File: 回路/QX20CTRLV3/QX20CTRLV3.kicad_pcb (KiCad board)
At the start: 2 copper layers, 56 x 47 mm, 26 parts, among them J1 VH_CAN, J2 VH_CAN, J3 VH_SRV1, J4 VH_SRV2, J5 USART, J6 I2C, J7 Conn_01x05, SW2 SW_SPDT, U1 BP5293-33, U2 STM32F303K8Tx, U3 SN65HVD232

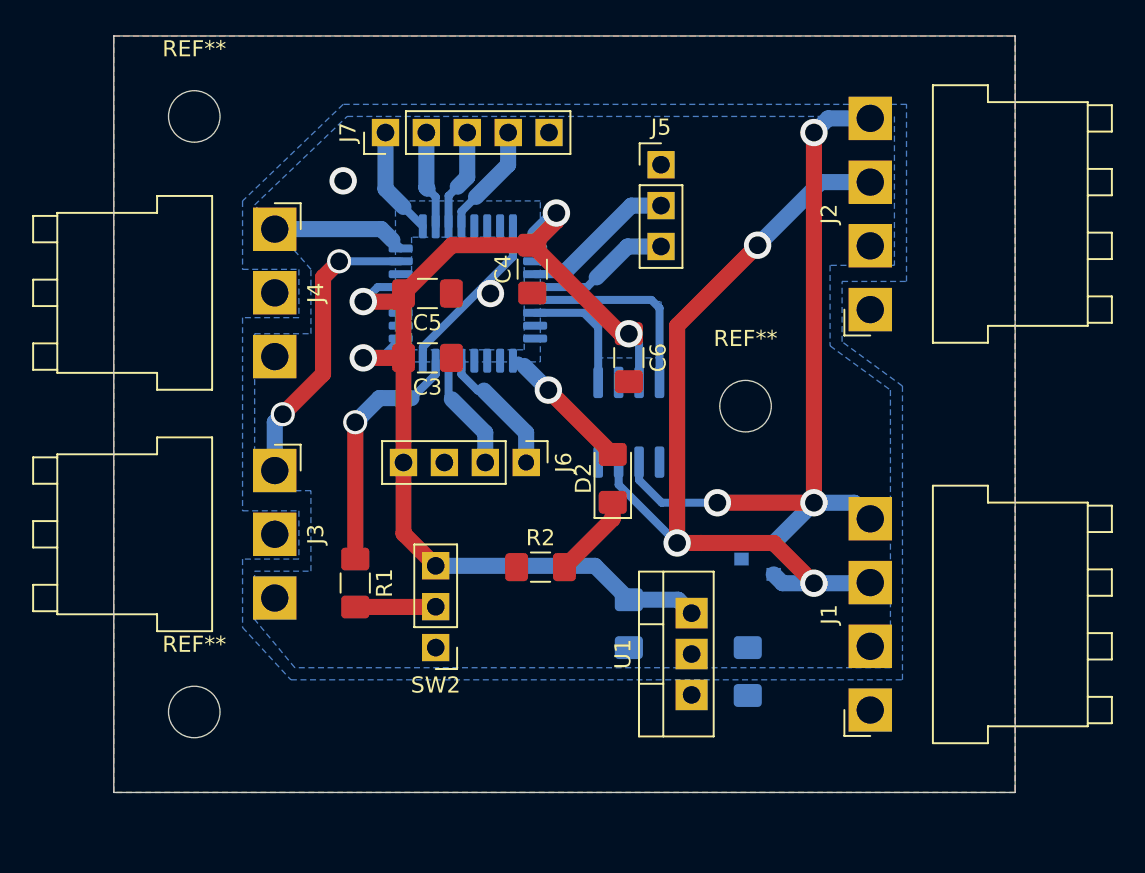
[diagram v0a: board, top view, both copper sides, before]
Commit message: QX20CTRLV3発注仕様
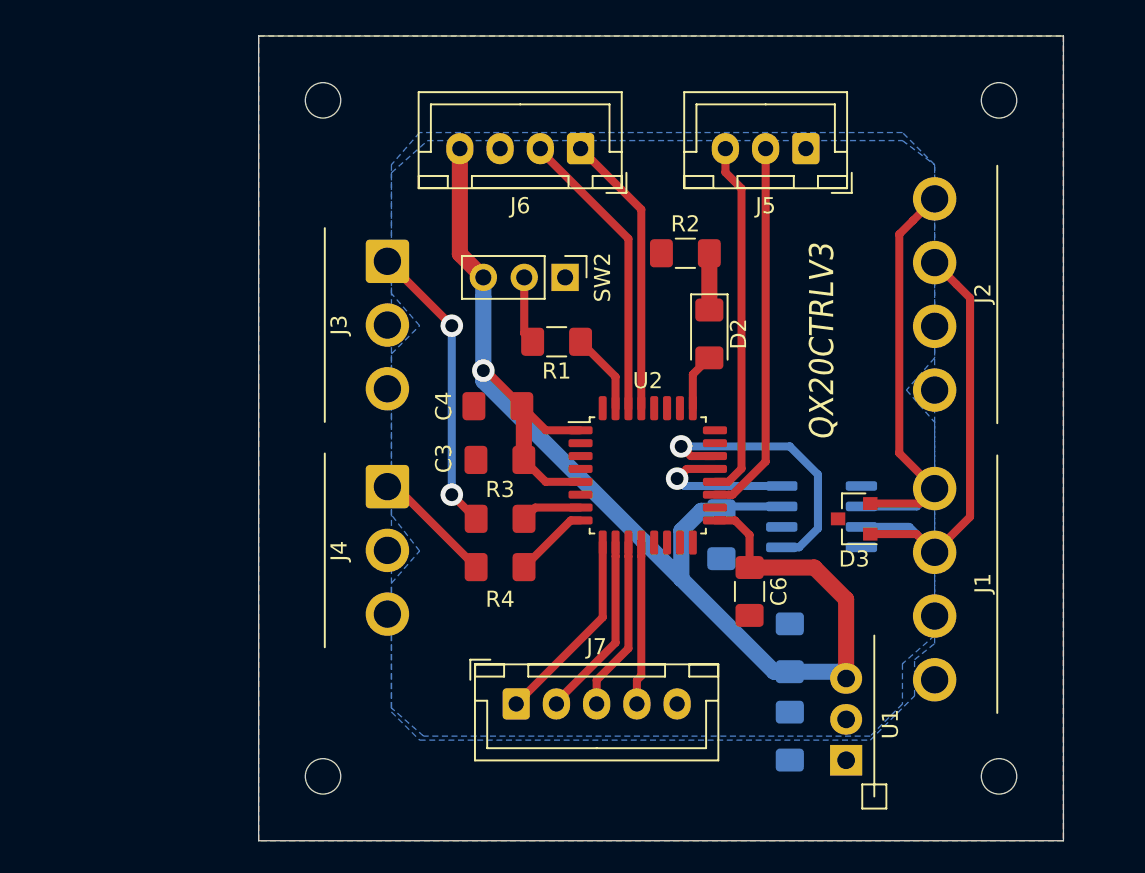
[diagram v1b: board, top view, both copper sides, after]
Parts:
- removed the ? at (151.0, 58.0)
- removed the ? at (152.0, 60.0)
- removed REF** (x3): MountingHole_3.2mm_M3, MountingHole:MountingHole_3.2mm_M3
- added ?: MountingHole_2.2mm_M2_DIN965, MountingHole:MountingHole_2.2mm_M2_DIN965, F.Cu at (104.0, 54.0)
- added ?: MountingHole_2.2mm_M2_DIN965, MountingHole:MountingHole_2.2mm_M2_DIN965, F.Cu at (104.0, 96.0)
- added ?: MountingHole_2.2mm_M2_DIN965, MountingHole:MountingHole_2.2mm_M2_DIN965, F.Cu at (146.0, 96.0)
- added ?: MountingHole_2.2mm_M2_DIN965, MountingHole:MountingHole_2.2mm_M2_DIN965, F.Cu at (146.0, 54.0)
- added R3: 0, Resistor_SMD:R_1206_3216Metric_Pad1.42x1.75mm_HandSolder, F.Cu at (115.0, 80.0)
- added R4: 0, Resistor_SMD:R_1206_3216Metric_Pad1.42x1.75mm_HandSolder, F.Cu at (115.0, 83.0)
- C5: moved to B.Cu
- D3, U2: moved to F.Cu
- J5: footprint Connector_PinHeader_2.54mm:PinHeader_1x03_P2.54mm_Vertical -> Connector_JST:JST_XH_B3B-XH-A_1x03_P2.50mm_Vertical
- J6: footprint Connector_PinHeader_2.54mm:PinHeader_1x04_P2.54mm_Vertical -> Connector_JST:JST_XH_B4B-XH-A_1x04_P2.50mm_Vertical
- J7: footprint Connector_PinHeader_2.54mm:PinHeader_1x05_P2.54mm_Vertical -> Connector_JST:JST_XH_B5B-XH-A_1x05_P2.50mm_Vertical
- moved J7 36.4 mm to (116.0, 91.5), turned to 0 degrees
- moved SW2 24.4 mm to (119.0, 65.0), turned to 270 degrees
- moved C5 23.6 mm to (128.8, 81.0), turned to 90 degrees
- moved R2 21.5 mm to (126.5, 63.5)
- moved J6 19.8 mm to (120.0, 57.0), turned to 180 degrees
- moved R1 19.5 mm to (118.5, 69.0), turned to 180 degrees
- moved J4 17.5 mm to (108.0, 78.0)
- moved C6 16.3 mm to (130.5, 84.5)
- moved U2 15.9 mm to (124.2, 77.3)
- moved J3 14.8 mm to (108.0, 64.0)
- moved U3 13.3 mm to (135.0, 79.9), turned to 0 degrees
- moved D2 10.8 mm to (128.0, 68.5), turned to 270 degrees
- moved U1 10.4 mm to (136.5, 95.0)
- moved C2 10.1 mm to (133.0, 88.0), turned to 90 degrees
- moved J5 9.06 mm to (134.0, 57.0), turned to 180 degrees
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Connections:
- D3 pad 1: CANL -> CANH
- D3 pad 2: CANH -> CANL
- J3 pad 1: PWM1 -> Net-(J3-Pad1)
- J4 pad 1: PWM2 -> Net-(J4-Pad1)
- U2 pad 13: Net-(U2-Pad13) -> (no net)
- U2 pad 14: Net-(U2-Pad14) -> (no net)
- U2 pad 15: Net-(U2-Pad15) -> (no net)
- U2 pad 18: Net-(U2-Pad18) -> (no net)
- U2 pad 2: Net-(U2-Pad2) -> (no net)
- U2 pad 23: Net-(U2-Pad23) -> (no net)
- U2 pad 24: Net-(U2-Pad24) -> (no net)
- U2 pad 26: Net-(U2-Pad26) -> (no net)
- U2 pad 27: Net-(U2-Pad27) -> (no net)
- U2 pad 28: Net-(U2-Pad28) -> (no net)
- U2 pad 3: Net-(U2-Pad3) -> (no net)
- U2 pad 4: Net-(U2-Pad4) -> (no net)
- U2 pad 6: Net-(U2-Pad6) -> (no net)
- U3 pad 5: Net-(U3-Pad5) -> (no net)
- U3 pad 8: Net-(U3-Pad8) -> (no net)
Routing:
- net CANH: track 51.5 -> 29.5 mm, vias 3 -> 0
- net Net-(J3-Pad1): track 0.00 -> 18.3 mm, vias 0 -> 2
- net CANL: track 46.9 -> 29.2 mm, vias 3 -> 0
- net PWM1: track 18.5 -> 3.80 mm, vias 2 -> 0
- net 3.3V: track 71.8 -> 86.4 mm, vias 4 -> 1
- net USART_TX: track 9.79 -> 23.4 mm
- net USART_RX: track 8.87 -> 22.3 mm
- net I2C_SDA: track 7.27 -> 18.4 mm
- net GND: track 10.8 -> 0.00 mm, vias 2 -> 0
- net Net-(R1-Pad1): track 15.6 -> 5.03 mm, vias 1 -> 0
- net CAN_TX: track 7.72 -> 17.7 mm, vias 0 -> 1
- net I2C_SCL: track 8.22 -> 17.7 mm
- net Net-(J4-Pad1): track 0.00 -> 7.58 mm
- net Net-(J7-Pad2): track 6.07 -> 11.5 mm
- net Net-(J7-Pad1): track 6.79 -> 12.3 mm
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- removed copper zone on B.Cu, net 3.3V
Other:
- board size 56 x 47 mm -> 50 x 50 mm
- net class 3.3V: via_dia 1.5 -> 1.4; via_drill 1.1 -> 0.8
- net class Default: via_dia 1.5 -> 1.4; via_drill 1.1 -> 0.8
- net class Power: via_dia 1.5 -> 1.4; via_drill 1.1 -> 0.8
- net class Wide: via_dia 1.5 -> 1.4; via_drill 1.1 -> 0.8
- rule pad_to_mask_clearance: 0.051 -> 0.1
- rule solder_mask_min_width: 0.25 -> 0.1
- rule via_min_drill: 1.1 -> 0.8
- rule via_min_size: 1.5 -> 1
- board text added: "QX20CTRLV3"
